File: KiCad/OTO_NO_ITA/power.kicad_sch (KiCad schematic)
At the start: 8 parts, among them U10 AP2127N-1.8TRG1, U9 AP7361EA-33E-13

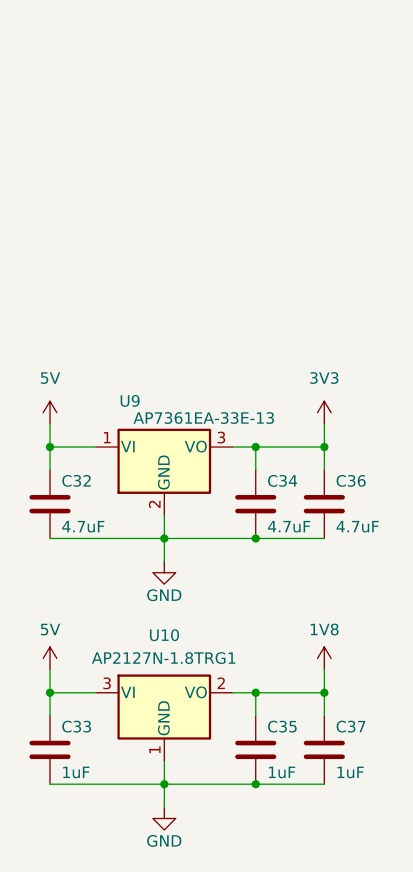
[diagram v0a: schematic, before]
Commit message: Updated schematics.
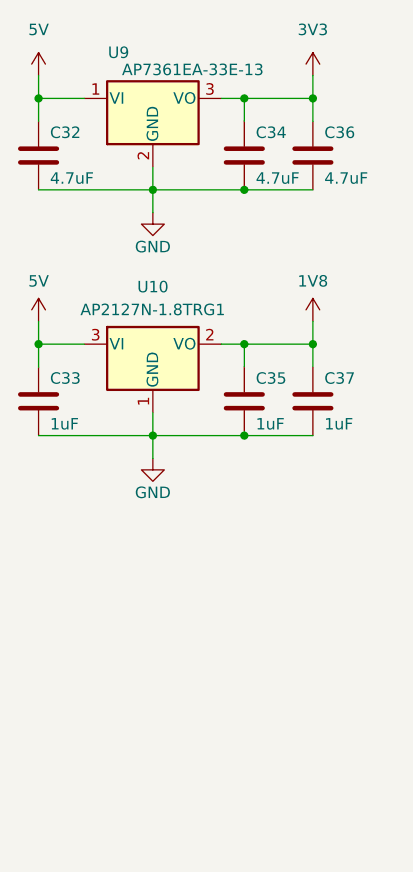
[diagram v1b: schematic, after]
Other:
- moved on the sheet: C32, C33, C34, C35, C36, C37, U10, U9
